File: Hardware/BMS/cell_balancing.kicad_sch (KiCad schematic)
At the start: 1 part, among them J1 Conn_02x09_Counter_Clockwise

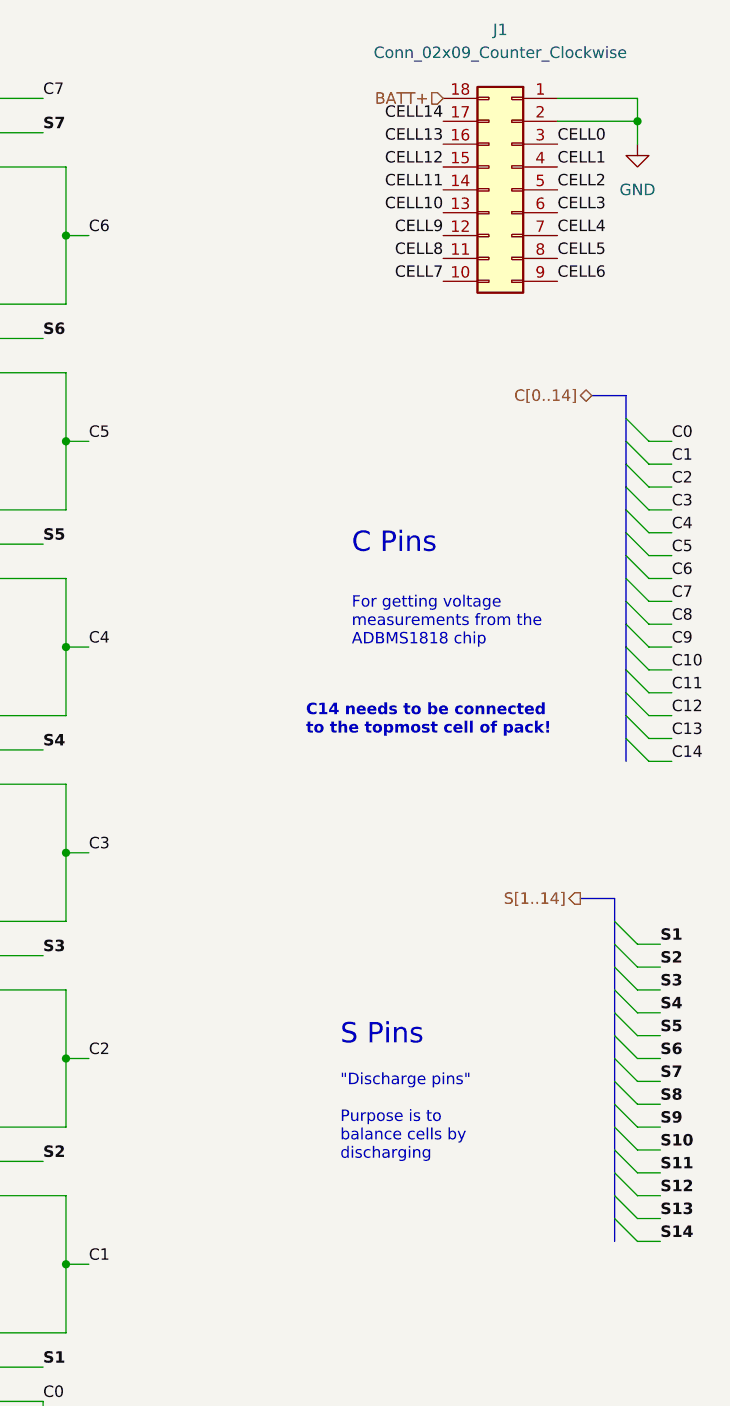
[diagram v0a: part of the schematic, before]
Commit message: edits to the BMS
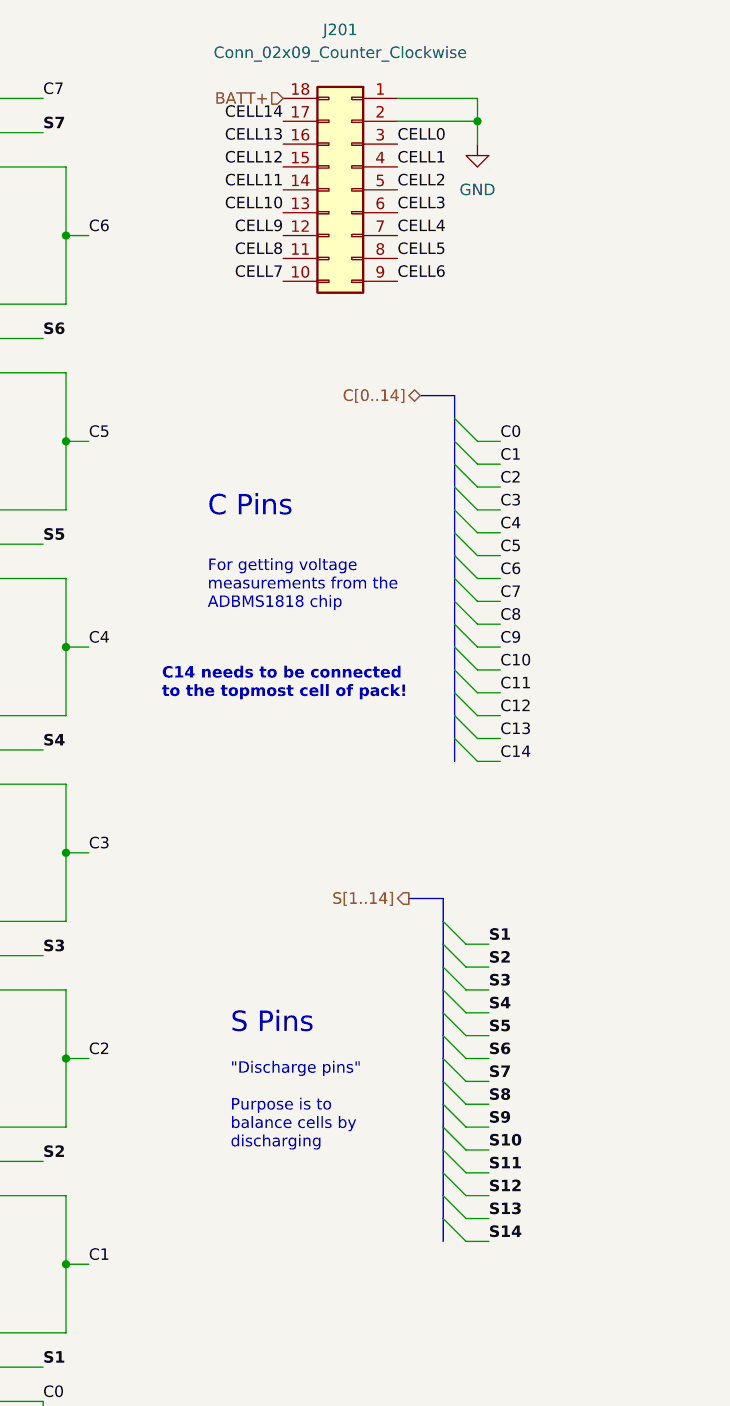
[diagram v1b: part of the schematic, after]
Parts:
- renumbered J1 to J201
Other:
- moved on the sheet: J201
